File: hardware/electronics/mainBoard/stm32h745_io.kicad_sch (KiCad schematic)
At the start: 14 parts, among them SW1 VAL, SW2 VAL, U1 STM32H745ZIT6, U20 TCAN1057A-Q1

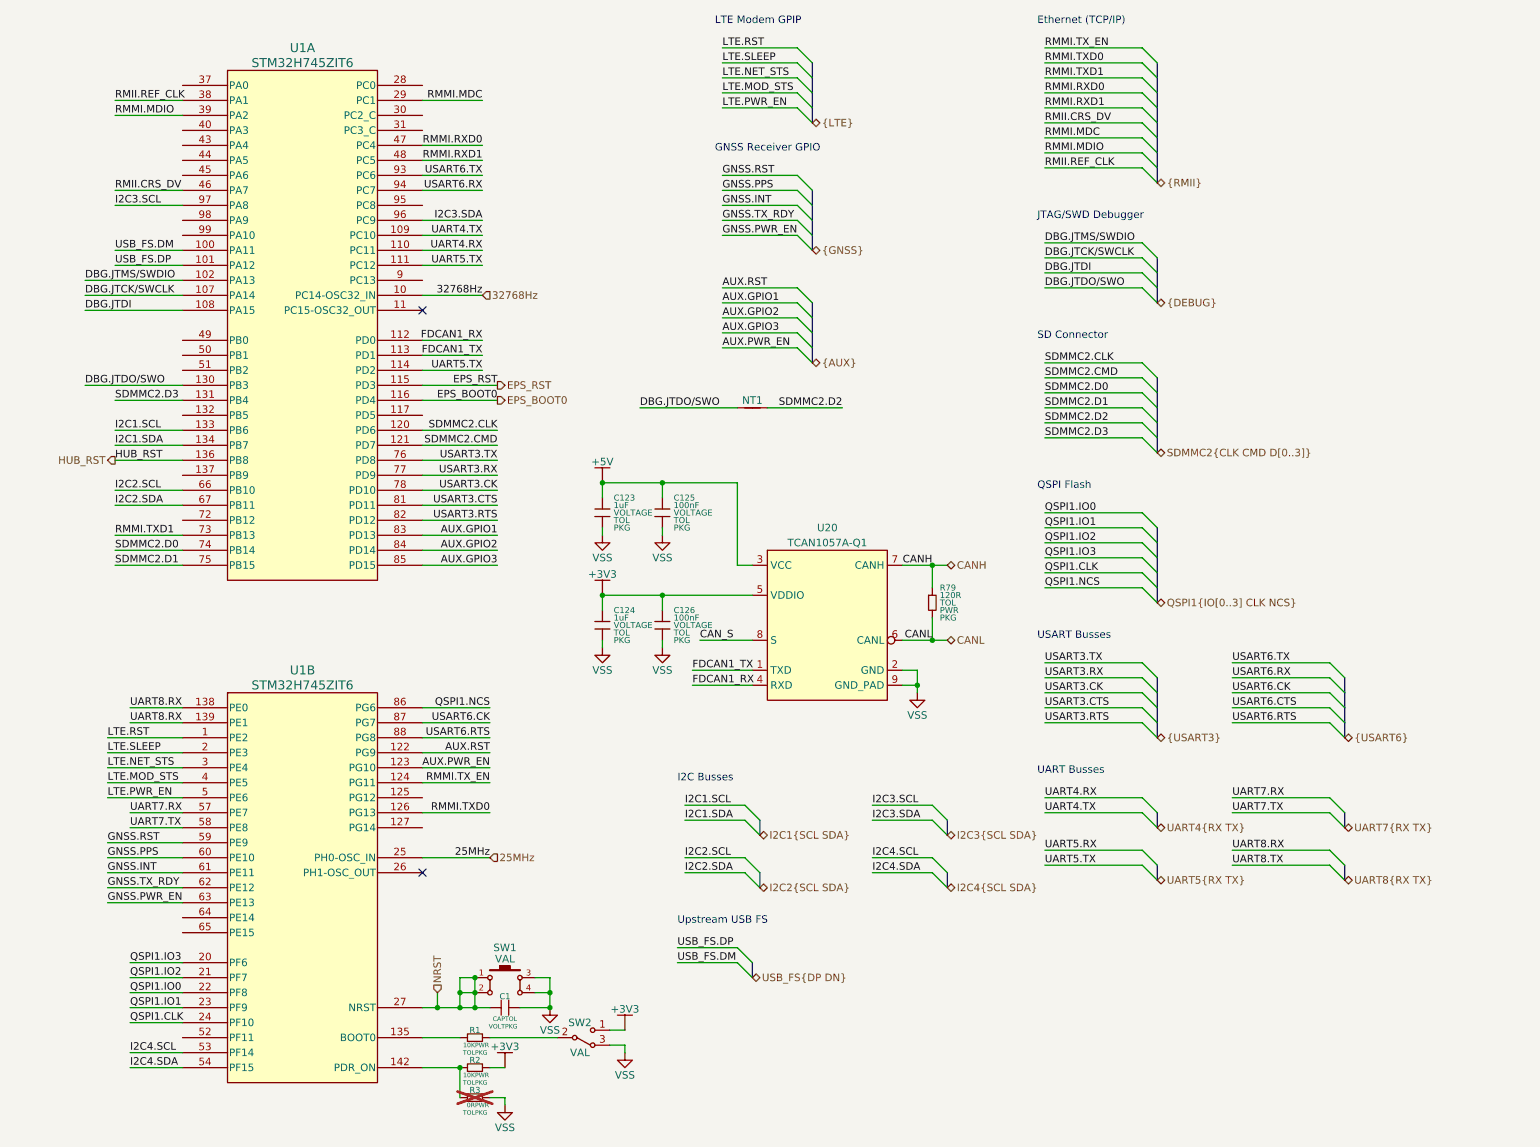
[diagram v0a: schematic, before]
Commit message: fixed nets
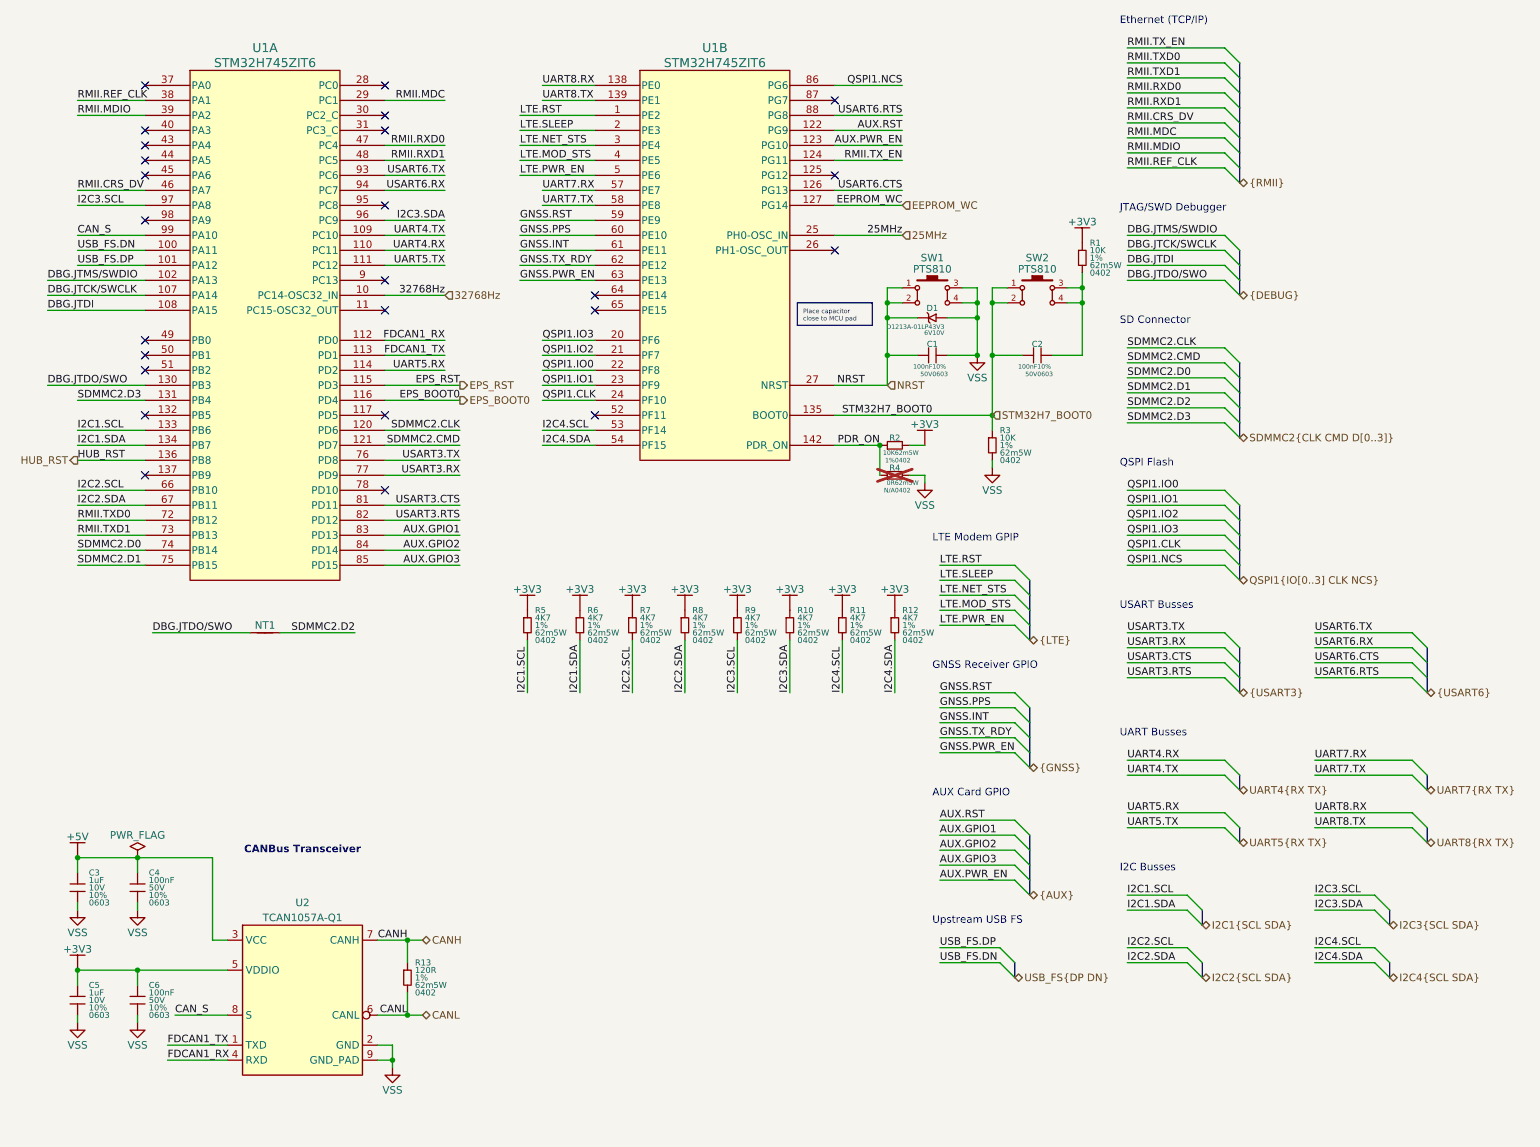
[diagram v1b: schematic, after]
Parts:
- removed C124: 1uF, symbol lib_sch:C
- removed C126: 100nF, symbol lib_sch:C
- removed R1: 10K, symbol lib_sch:R_horizontal
- removed SW2: VAL, symbol lib_sch:SPDT
- added C2: 100nF, symbol lib_sch:C_horizontal
- added C5: 1uF, symbol lib_sch:C
- added C6: 100nF, symbol lib_sch:C
- added D1: D1213A-01LP4, symbol lib_sch:D_TVS_single_horizontal
- added R1, R3: 10K, symbol lib_sch:R
- added R10, R11, R12, R5, R6, R7, R8, R9: 4K7, symbol lib_sch:R
- added SW2: PTS810, symbol lib_sch:SPST-NO Button
- C1: value CAP -> 100nF; DKPN (none) -> 478-KAM15AR71H104KTCT-ND; MPN (none) -> 06035C104K4T2A; Manufacturer (none) -> KYOCERA AVX; Package PKG -> 0603; Tolerace TOL -> (none); Tolerance (none) -> 10%; Voltage Rating VOLT -> 50V
- C3: renamed from C123; DKPN (none) -> 478-KAM15AR71A105KTCT-ND; MPN (none) -> KAM15AR71A105KT; Manufacturer (none) -> KYOCERA AVX; Package PKG -> 0603; Tolerance TOL -> 10%; Voltage Rating VOLTAGE -> 10V
- C4: renamed from C125; DKPN (none) -> 478-KAM15AR71H104KTCT-ND; MPN (none) -> 06035C104K4T2A; Manufacturer (none) -> KYOCERA AVX; Package PKG -> 0603; Tolerance TOL -> 10%; Voltage Rating VOLTAGE -> 50V
- R13: renamed from R79; DKPN (none) -> 541-120LCT-ND; MPN (none) -> CRCW0402120RFKED; Manufacturer (none) -> Vishay Dale; Package PKG -> 0402; Power Rating PWR -> 62m5W; Tolerance TOL -> 1%
- R2: DKPN (none) -> 541-10.0KLCT-ND; MPN (none) -> CRCW040210K0FKED; Manufacturer (none) -> Vishay Dale; Package PKG -> 0402; Power Rating PWR -> 62m5W; Tolerance TOL -> 1%
- R4: renamed from R3; DKPN (none) -> 541-0.0JCT-ND; MPN (none) -> CRCW04020000Z0ED; Manufacturer (none) -> Vishay Dale; Package PKG -> 0402; Power Rating PWR -> 62m5W; Tolerance TOL -> N/A
- SW1: value VAL -> PTS810; DKPN (none) -> CKN10502CT-ND; MPN (none) -> PTS810SJM250SMTR LFS; Manufacturer (none) -> C&K
- U1: footprint LQFP-144 -> (none); DKPN (none) -> 497-19501-ND; MPN (none) -> STM32H745ZIT6; Manufacturer (none) -> STMicroelectronics
- U2: renamed from U20; symbol .DS-RF-Tranceivers-and-Modems:TCAN1057A-Q1 -> lib_sch:TCAN1057A-Q1; DKPN (none) -> 296-TCAN1057ADRBRQ1CT-ND; MPN (none) -> TCAN1057ADRBRQ1
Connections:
- net RMMI.TXD0 is gone; now on net USART6.CTS: U1.126 (PG13)
- net +3V3: now also C5.1, C6.1, R1.1, R10.1, R11.1, R12.1, R5.1, R6.1, R7.1, R8.1, R9.1
- net CAN_S: now also U1.99 (PA10)
- net I2C1.SCL: now also R5.2
- net I2C1.SDA: now also R6.2
- net I2C2.SCL: now also R7.2
- net I2C2.SDA: now also R8.2
- net I2C3.SCL: now also R9.2
- net I2C3.SDA: now also R10.2
- net I2C4.SCL: now also R11.2
- net I2C4.SDA: now also R12.2
- net NRST: now also D1.2
- net UART5.RX: now also U1.114 (PD2)
- net UART5.TX: no longer U1.114 (PD2)
- net UART8.RX: no longer U1.139 (PE1)
- net UART8.TX: now also U1.139 (PE1)
- net VSS: now also C5.2, C6.2, D1.1, R3.2
- net EEPROM_WC: now reaches U1.127 (PG14)
- net STM32H7_BOOT0: now reaches U1.135 (BOOT0)
- net STM32H7_BOOT0: now also C2.1, R3.1, SW2.1, SW2.2
- net PDR_ON: now reaches R2.1, R4.1, U1.142 (PDR_ON)
- net RMII.TXD0: now reaches U1.72 (PB12)
- net RMMI.MDC renamed RMII.MDC
- net RMMI.MDIO renamed RMII.MDIO
- net RMMI.RXD0 renamed RMII.RXD0
- net RMMI.RXD1 renamed RMII.RXD1
- net RMMI.TXD1 renamed RMII.TXD1
- net RMMI.TX_EN renamed RMII.TX_EN
- net USART3.CK: no longer names the net of U1.78 (PD10)
- net USART6.CK: no longer names the net of U1.87 (PG7)
- net USB_FS.DM renamed USB_FS.DN
- new net: C2.2, R1.2, SW2.3, SW2.4
- no-connect marks 2 -> 25
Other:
- note added: "AUX Card GPIO"
- note added: "CANBus Transceiver"
- moved on the sheet: C1, C3, C4, NT1, R13, R2, R4, SW1, U1A, U1B, U2
